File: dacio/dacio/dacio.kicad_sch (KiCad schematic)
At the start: 56 parts, among them J3 RJ45_Shielded, J4 RJ45_Shielded, J5 Conn_02x12_Odd_Even, U1 SN74LVC1T45DBV, U10 MAX3232, U11 MAX3232, U12 74HCT32D, U13 74HCT00D, U14 74HCT32D, U15 74HCT00D, U16 TLV70033_SOT353, U17 SN74LV8T374PWR, U18 SN74LV8T374PWR, U2 SN74LVC1T45DBV, U3 TLV70018_SOT353, U4 MAX487CSA+, U5 MAX487CSA+, U6 MAX487CSA+, U7 MAX487CSA+, U8 MAX487CSA+, U9 MAX487CSA+

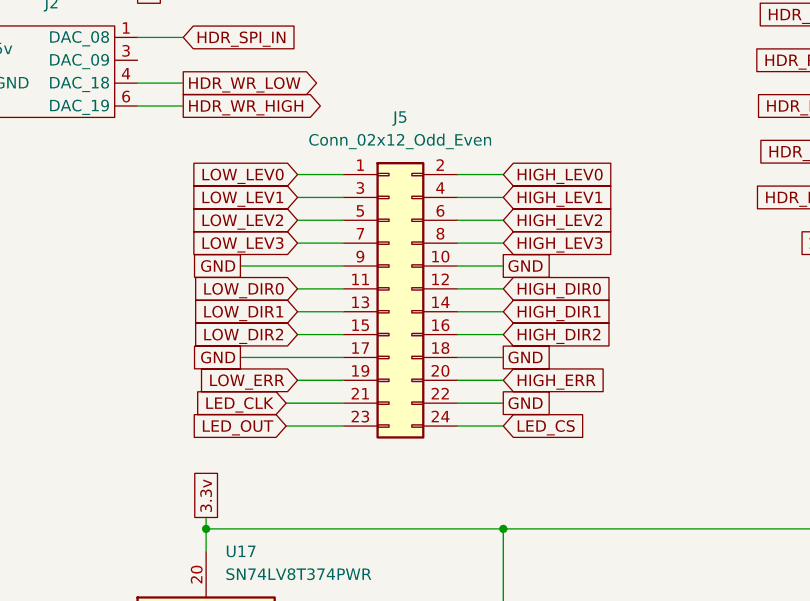
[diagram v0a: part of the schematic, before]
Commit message: Fixed some of the layout.
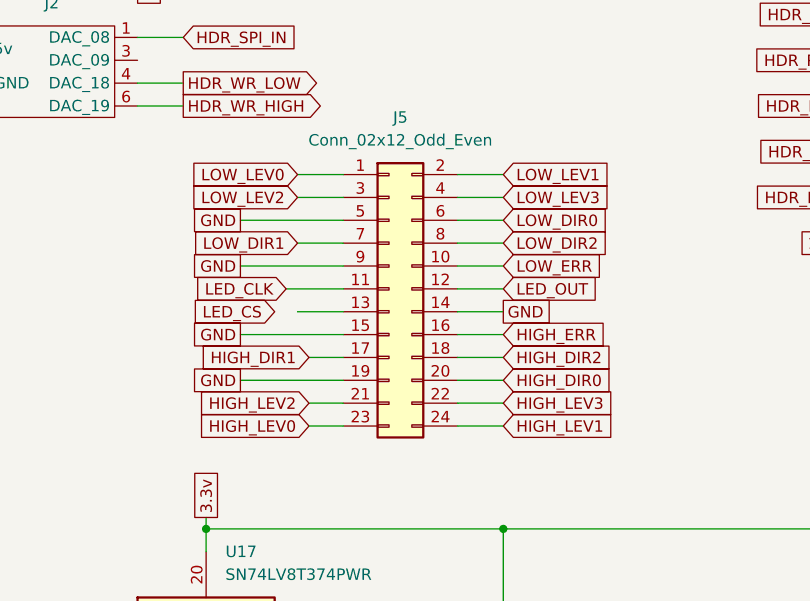
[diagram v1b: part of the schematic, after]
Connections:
- net GND: now also J5.14 (Pin_14), J5.15 (Pin_15), J5.19 (Pin_19), J5.5 (Pin_5); no longer J5.10 (Pin_10), J5.17 (Pin_17), J5.18 (Pin_18), J5.22 (Pin_22)
- net HIGH_DIR0: now also J5.20 (Pin_20); no longer J5.12 (Pin_12)
- net HIGH_DIR1: now also J5.17 (Pin_17); no longer J5.14 (Pin_14)
- net HIGH_DIR2: now also J5.18 (Pin_18); no longer J5.16 (Pin_16)
- net HIGH_ERR: now also J5.16 (Pin_16); no longer J5.20 (Pin_20)
- net HIGH_LEV0: now also J5.23 (Pin_23); no longer J5.2 (Pin_2)
- net HIGH_LEV1: now also J5.24 (Pin_24); no longer J5.4 (Pin_4)
- net HIGH_LEV2: now also J5.21 (Pin_21); no longer J5.6 (Pin_6)
- net HIGH_LEV3: now also J5.22 (Pin_22); no longer J5.8 (Pin_8)
- net LED_CLK: now also J5.11 (Pin_11); no longer J5.21 (Pin_21)
- net LED_CS: no longer J5.24 (Pin_24)
- net LED_OUT: now also J5.12 (Pin_12); no longer J5.23 (Pin_23)
- net LOW_DIR0: now also J5.6 (Pin_6); no longer J5.11 (Pin_11)
- net LOW_DIR1: now also J5.7 (Pin_7); no longer J5.13 (Pin_13)
- net LOW_DIR2: now also J5.8 (Pin_8); no longer J5.15 (Pin_15)
- net LOW_ERR: now also J5.10 (Pin_10); no longer J5.19 (Pin_19)
- net LOW_LEV1: now also J5.2 (Pin_2); no longer J5.3 (Pin_3)
- net LOW_LEV2: now also J5.3 (Pin_3); no longer J5.5 (Pin_5)
- net LOW_LEV3: now also J5.4 (Pin_4); no longer J5.7 (Pin_7)
